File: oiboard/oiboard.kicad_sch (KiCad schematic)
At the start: 37 parts, among them J1 Conn_01x04, U1 LM324

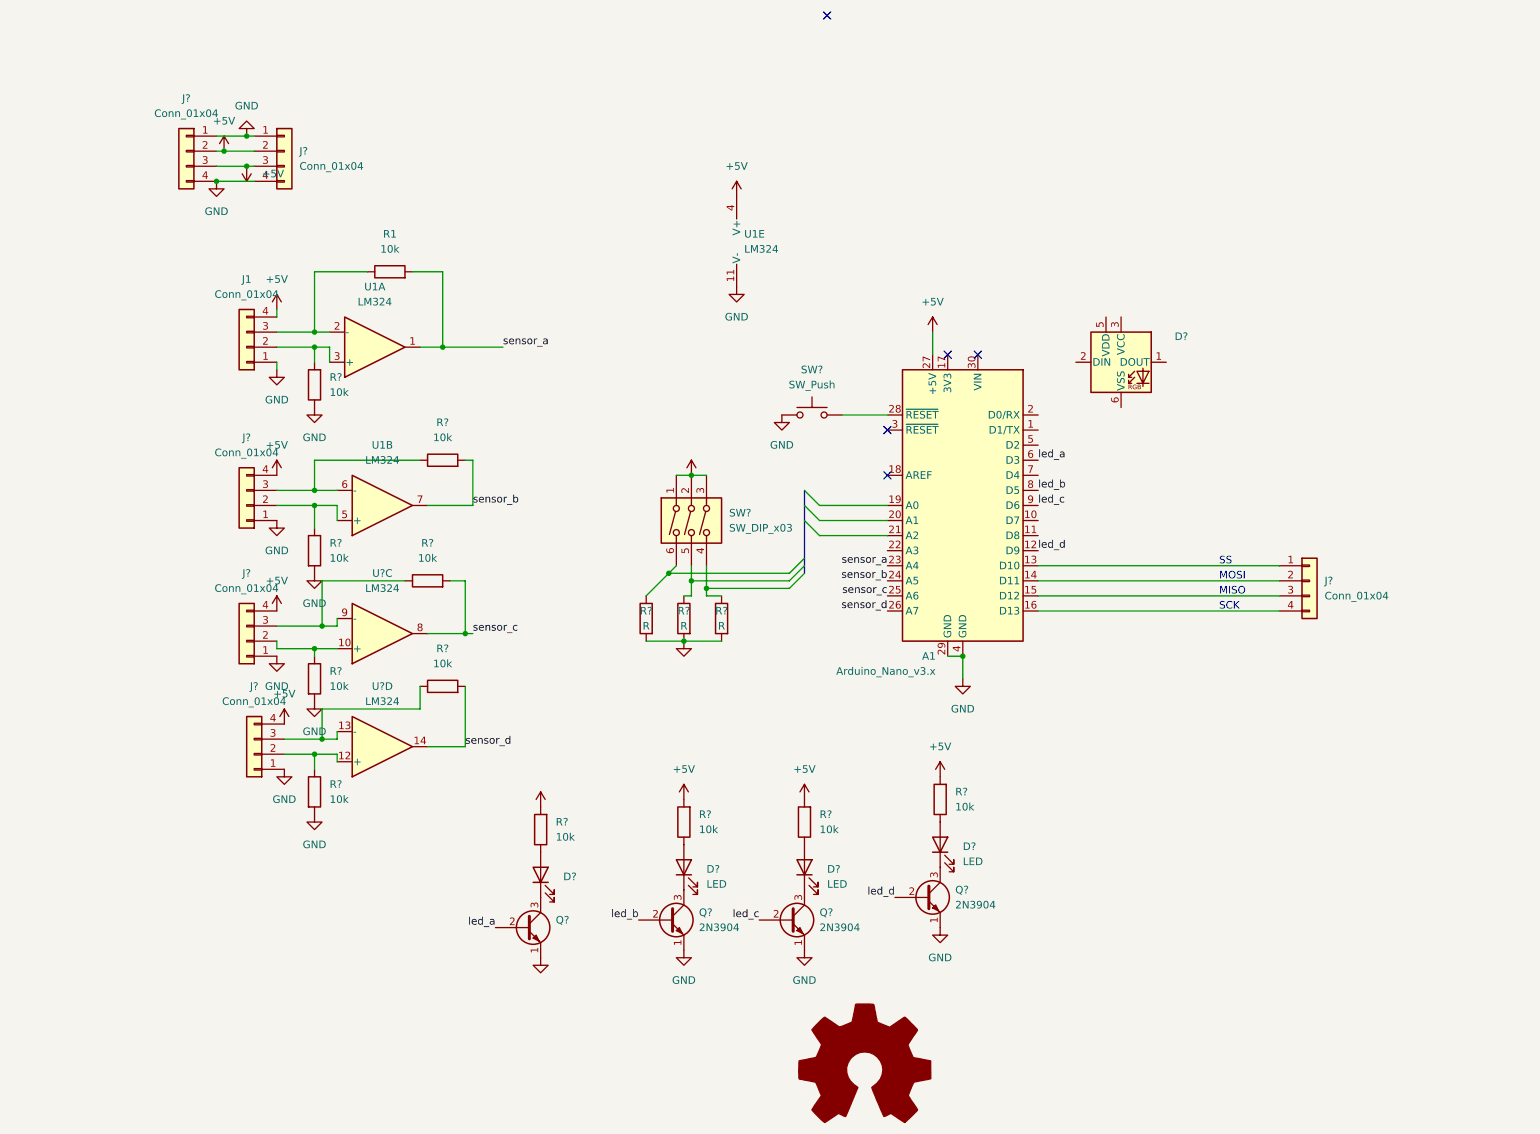
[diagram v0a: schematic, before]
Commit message: feat: finalize the board layout
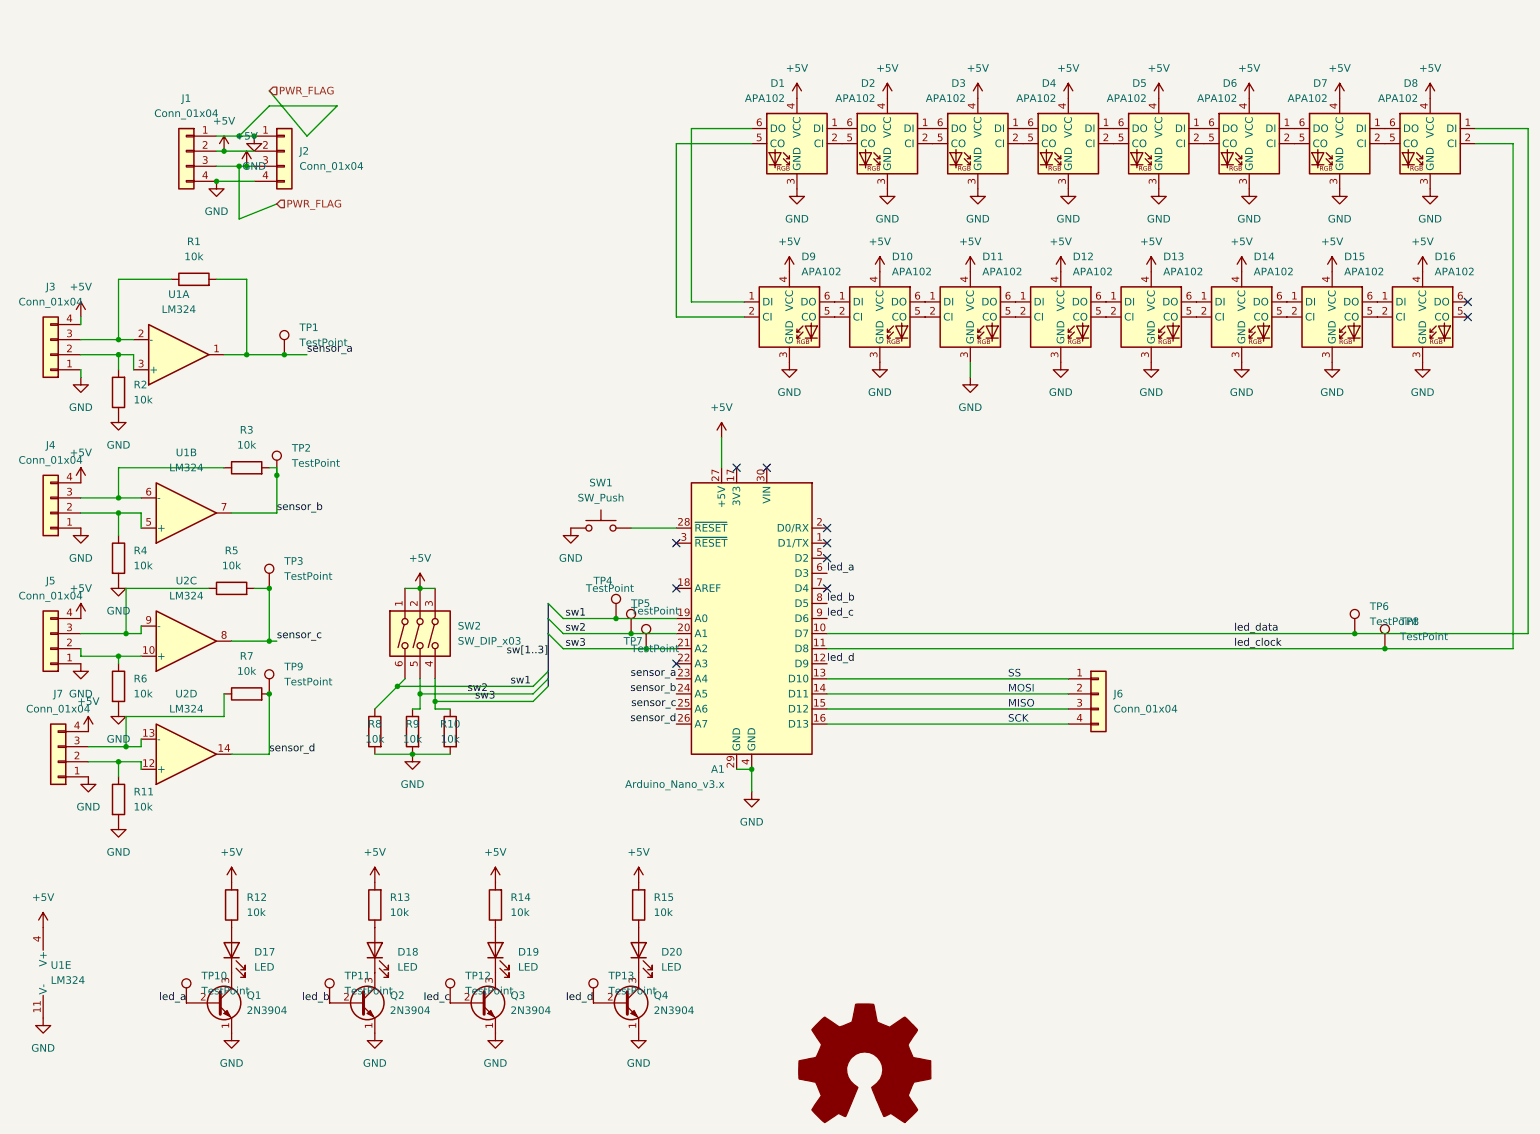
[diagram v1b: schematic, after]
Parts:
- removed D?: (no value), symbol LED:WS2812
- added D1, D10, D11, D12, D13, D14, D15, D16, D2, D3, D4, D5, D6, D7, D8, D9: APA102, LED_SMD:LED_RGB_5050-6, symbol LED:APA102
- added TP1, TP10, TP11, TP12, TP13, TP2, TP3, TP4, TP5, TP6, TP7, TP8, TP9: TestPoint, TestPoint:TestPoint_THTPad_D1.5mm_Drill0.7mm, symbol Connector:TestPoint
- D17: renamed from D?; value (none) -> LED; footprint (none) -> LED_THT:LED_D5.0mm
- D18, D19, D20: renamed from D?; footprint (none) -> LED_THT:LED_D5.0mm
- Q1: renamed from Q?; value (none) -> 2N3904; footprint (none) -> Package_TO_SOT_THT:TO-92_Inline
- R1: footprint Resistor_THT:R_Axial_DIN0207_L6.3mm_D2.5mm_P15.24mm_Horizontal -> Resistor_THT:R_Axial_DIN0207_L6.3mm_D2.5mm_P10.16mm_Horizontal
- R10, R8, R9: renamed from R?; value R -> 10k; footprint (none) -> Resistor_THT:R_Axial_DIN0207_L6.3mm_D2.5mm_P10.16mm_Horizontal
- R11, R12, R13, R15, R2, R3, R4, R5, R6, R7: renamed from R?; footprint Resistor_THT:R_Axial_DIN0207_L6.3mm_D2.5mm_P15.24mm_Horizontal -> Resistor_THT:R_Axial_DIN0207_L6.3mm_D2.5mm_P10.16mm_Horizontal
- R14: renamed from R?; footprint Resistor_THT:R_Axial_DIN0207_L6.3mm_D2.5mm_P15.24mm_Horizontal -> Button_Switch_THT:SW_CuK_JS202011CQN_DPDT_Straight
- SW1: renamed from SW?; footprint (none) -> Button_Switch_THT:SW_PUSH_6mm
- SW2: renamed from SW?; footprint (none) -> Button_Switch_THT:SW_DIP_SPSTx03_Slide_9.78x9.8mm_W7.62mm_P2.54mm
- gave numbers to parts that had none: 10
- renumbered J1 to J3
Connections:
- net GND is gone; now on net +5V: A1.29 (GND), A1.4 (GND), J1.1 (Pin_1), J1.4 (Pin_4), J2.1 (Pin_1), J2.4 (Pin_4), J3.1 (Pin_1), J4.1 (Pin_1), J5.1 (Pin_1), J7.1 (Pin_1), Q1.1 (E), Q2.1 (E), Q3.1 (E), Q4.1 (E), R10.2, R11.2, R2.1, R4.2, R6.2, R8.2, R9.2, SW1.1, U1.11 (V-)
- net +5V: now also D1.3 (GND), D1.4 (VCC), D10.3 (GND), D10.4 (VCC), D11.3 (GND), D11.4 (VCC), D12.3 (GND), D12.4 (VCC), D13.3 (GND), D13.4 (VCC), D14.3 (GND), D14.4 (VCC), D15.3 (GND), D15.4 (VCC), D16.3 (GND), D16.4 (VCC), D2.3 (GND), D2.4 (VCC), D3.3 (GND), D3.4 (VCC), D4.3 (GND), D4.4 (VCC), D5.3 (GND), D5.4 (VCC), D6.3 (GND), D6.4 (VCC), D7.3 (GND), D7.4 (VCC), D8.3 (GND), D8.4 (VCC), D9.3 (GND), D9.4 (VCC)
- net led_a: now also TP10.1
- net led_b: now also TP11.1
- net led_c: now also TP12.1
- net led_d: now also TP13.1
- net sensor_a: now also TP1.1
- net sensor_b: now also TP2.1
- net sensor_c: now also TP3.1
- net sensor_d: now also TP9.1
- net sw3: now reaches R10.1, SW2.4
- net sw3: now also A1.21 (A2), TP7.1
- net led_data: now reaches A1.10 (D7)
- net led_data: now also D8.1 (DI), TP6.1
- net led_clock : now reaches A1.11 (D8)
- net led_clock : now also D8.2 (CI), TP8.1
- net sw1: now reaches A1.19 (A0)
- net sw1: now also R8.1, SW2.6, TP4.1
- net sw2: now reaches A1.20 (A1)
- net sw2: now also R9.1, SW2.5, TP5.1
- new net: D12.6 (DO), D13.1 (DI)
- new net: D12.5 (CO), D13.2 (CI)
- new net: D13.5 (CO), D14.2 (CI)
- new net: D13.6 (DO), D14.1 (DI)
- new net: D6.1 (DI), D7.6 (DO)
- new net: D6.2 (CI), D7.5 (CO)
- new net: D5.2 (CI), D6.5 (CO)
- new net: D5.1 (DI), D6.6 (DO)
- new net: D14.6 (DO), D15.1 (DI)
- new net: D14.5 (CO), D15.2 (CI)
- new net: D15.5 (CO), D16.2 (CI)
- new net: D15.6 (DO), D16.1 (DI)
- new net: D7.2 (CI), D8.5 (CO)
- new net: D7.1 (DI), D8.6 (DO)
- new net: D11.6 (DO), D12.1 (DI)
- new net: D11.5 (CO), D12.2 (CI)
- new net: D1.6 (DO), D9.1 (DI)
- new net: D1.5 (CO), D9.2 (CI)
- new net: D10.2 (CI), D9.5 (CO)
- new net: D10.1 (DI), D9.6 (DO)
- new net: D2.1 (DI), D3.6 (DO)
- new net: D2.2 (CI), D3.5 (CO)
- new net: D1.2 (CI), D2.5 (CO)
- new net: D1.1 (DI), D2.6 (DO)
- new net: D4.1 (DI), D5.6 (DO)
- new net: D4.2 (CI), D5.5 (CO)
- new net: D3.2 (CI), D4.5 (CO)
- new net: D3.1 (DI), D4.6 (DO)
- new net: D10.6 (DO), D11.1 (DI)
- new net: D10.5 (CO), D11.2 (CI)
- no-connect marks 5 -> 11
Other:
- moved on the sheet: A1, D17, D18, D19, D20, J3, J4, J5, J6, J7, Q1, Q2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
